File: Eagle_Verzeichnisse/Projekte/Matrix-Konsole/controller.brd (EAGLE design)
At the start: 114.3 x 63.2 mm, 21 parts, among them IC1 74HC165D

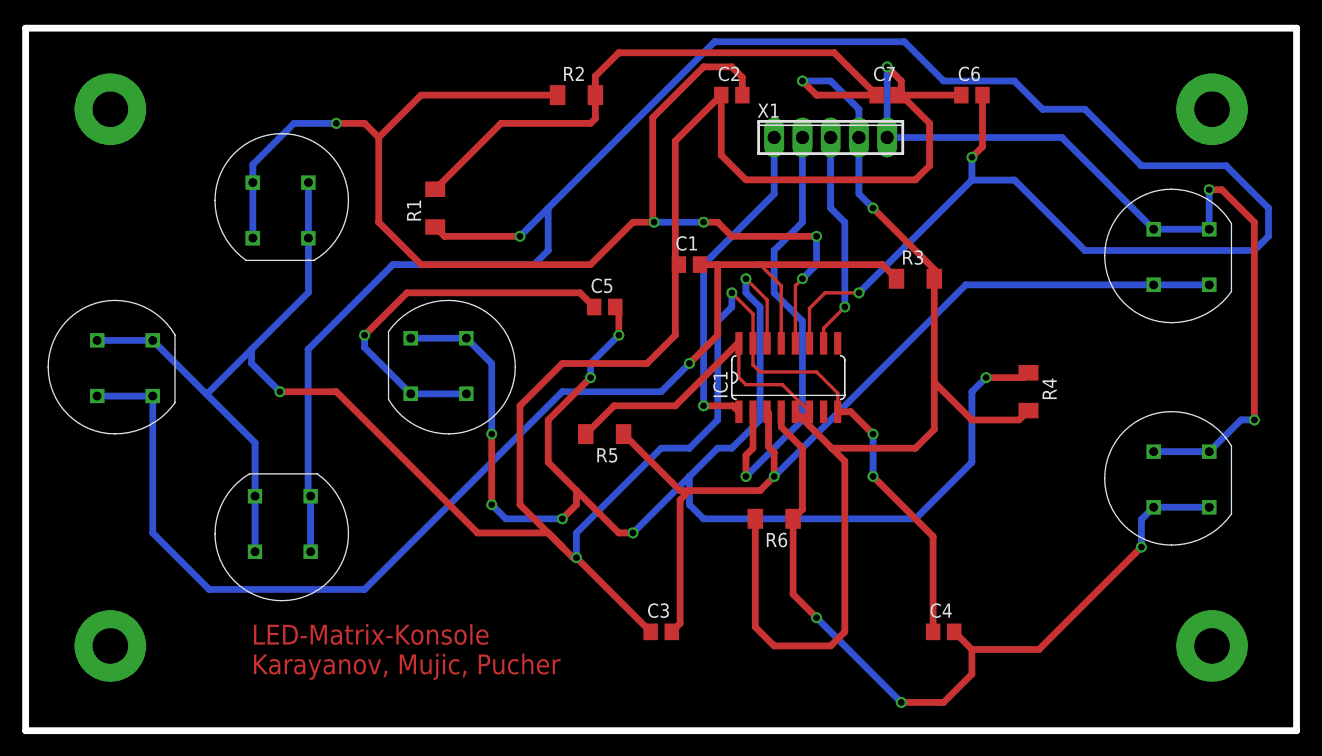
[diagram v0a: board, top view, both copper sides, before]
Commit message: Made final changes to the layout and added PDF-Files
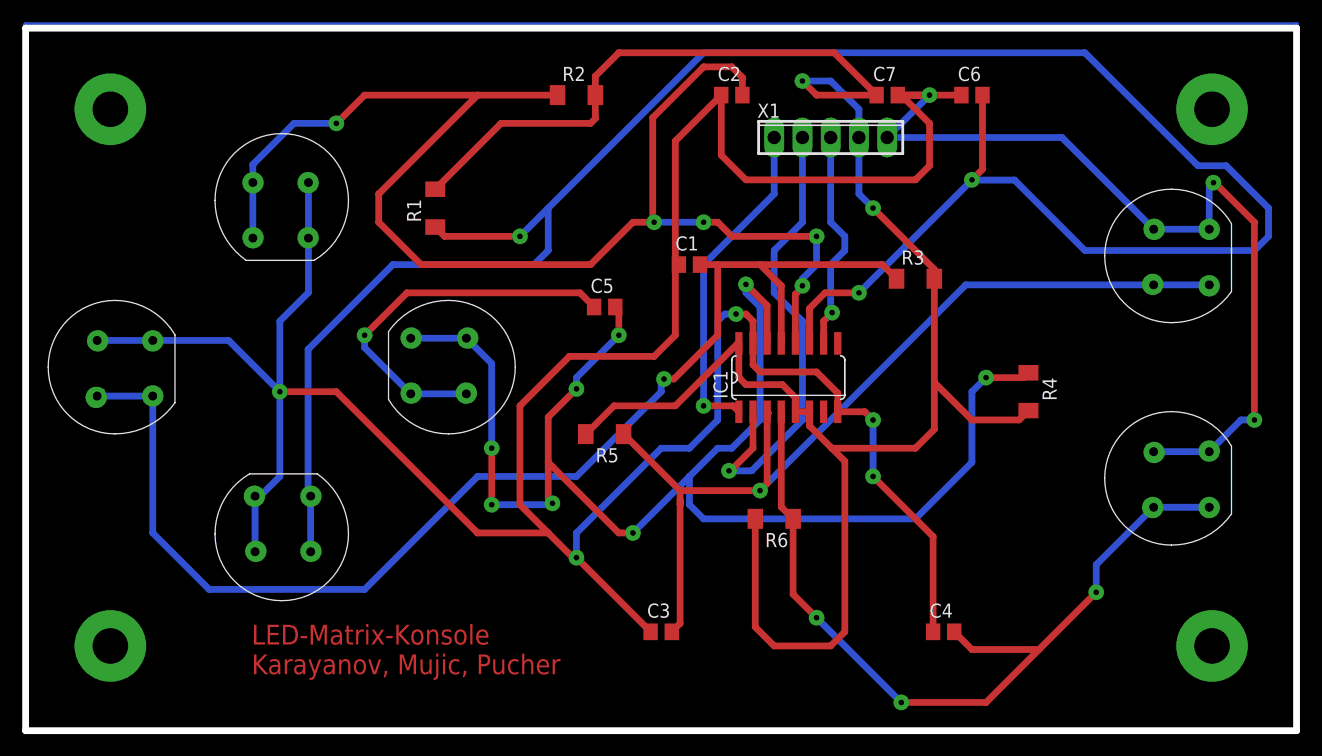
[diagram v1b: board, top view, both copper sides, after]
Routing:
- net N$8: track 0.00 -> 355.6 mm
- net D1: track 120.1 -> 126.6 mm
- net GND: track 342.4 -> 336.8 mm
- net D5: track 71.3 -> 75.3 mm
- net D3: track 136.0 -> 134.4 mm
- net D4: track 81.9 -> 83.4 mm
- net N$2: track 40.8 -> 42.3 mm
- net N$3: track 19.8 -> 21.3 mm
- net D0: track 199.0 -> 198.2 mm
- net 5V: track 183.0 -> 182.4 mm
- net D2: track 112.1 -> 112.6 mm
